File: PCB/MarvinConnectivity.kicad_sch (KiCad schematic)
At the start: 13 parts, among them J1 PROG / DBG, J10 EXP1, J11 EXP2, J2 EXPA, J3 EXPC, J4 SERVO POW 1, J5 SERVO POW 2, J6 EXPB, J7 EXPD, J8 SERVO SIG 1, J9 SERVO SIG 2

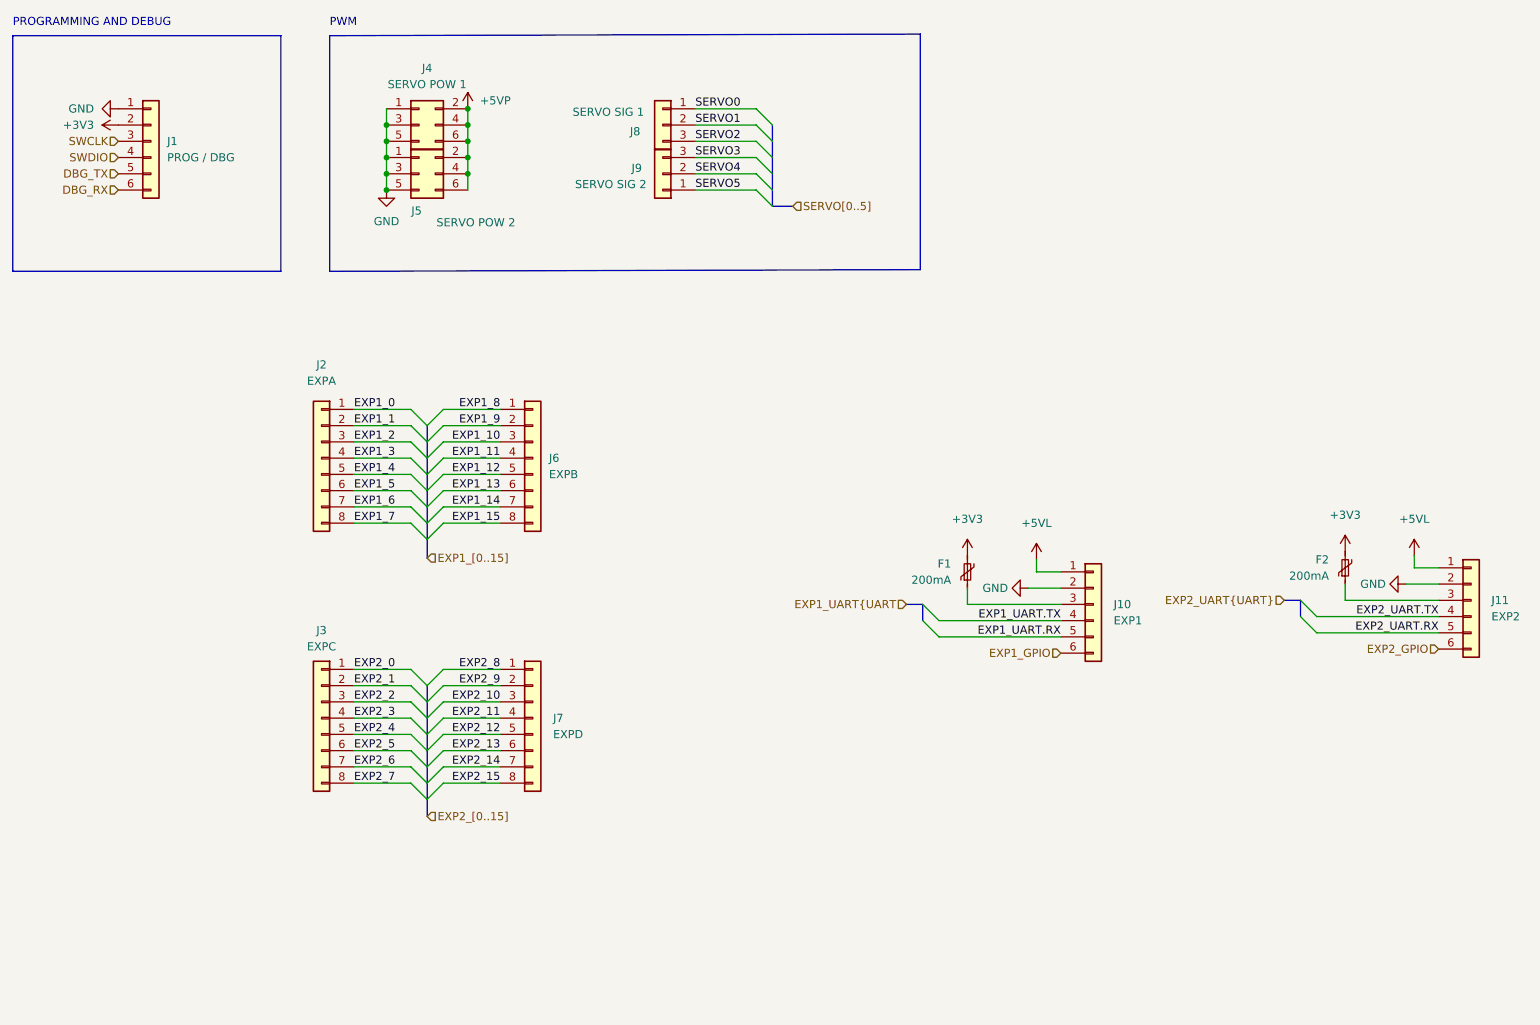
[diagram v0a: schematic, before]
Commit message: v2!
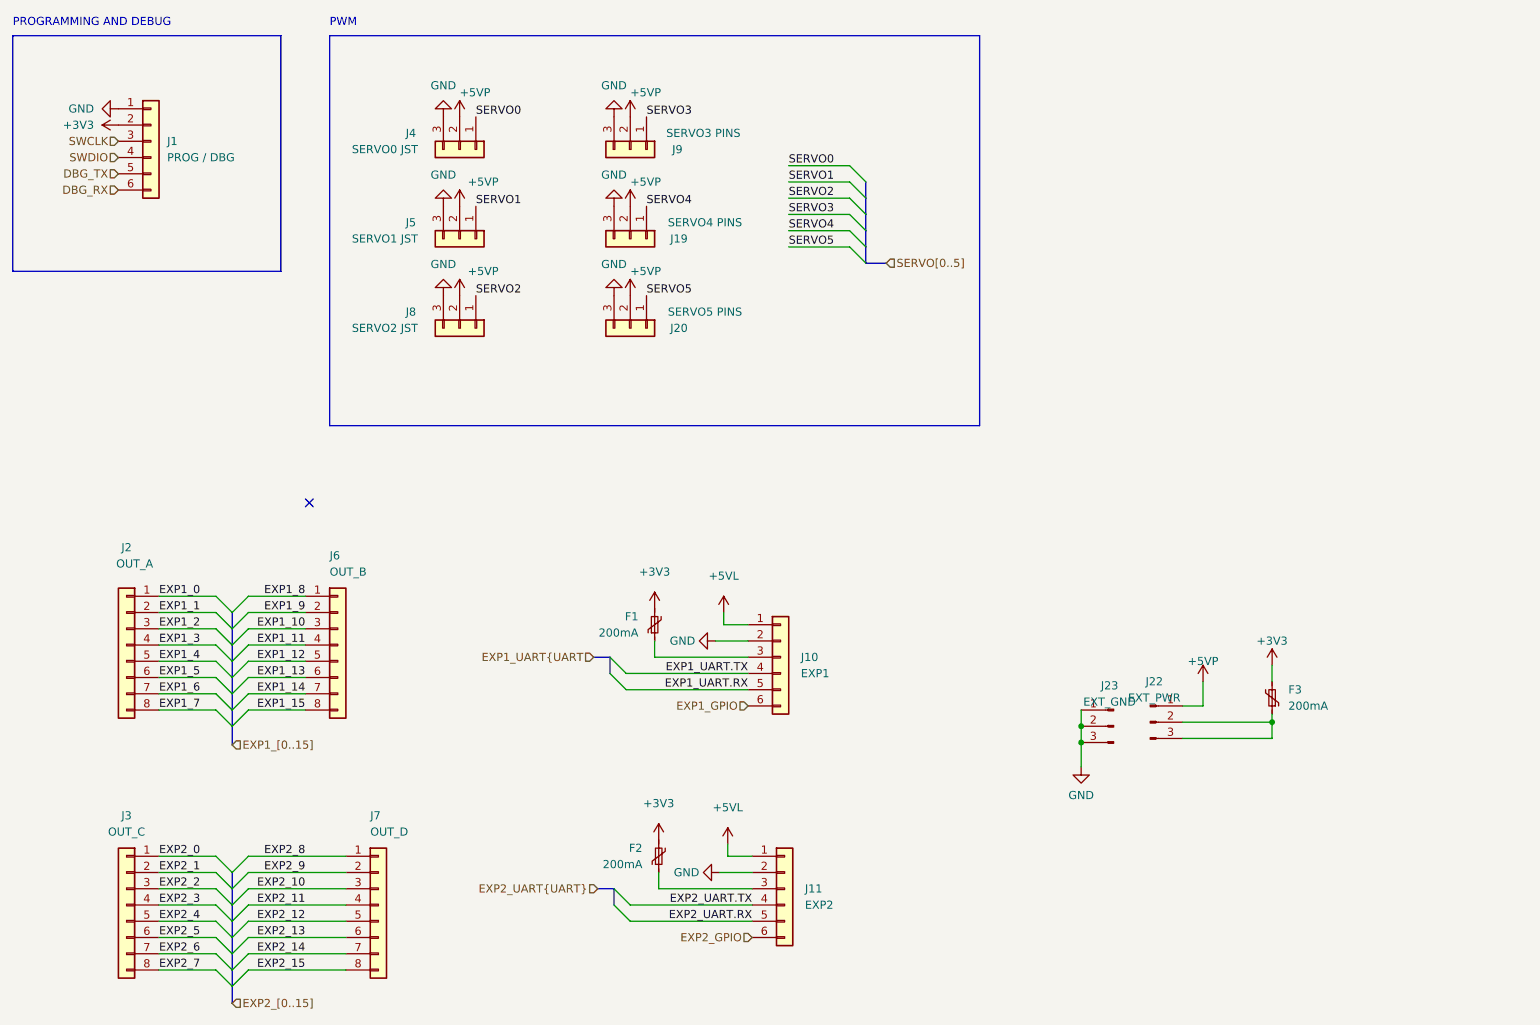
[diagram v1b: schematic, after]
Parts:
- removed J4: SERVO POW 1, Connector_PinHeader_2.54mm:PinHeader_2x03_P2.54mm_Vertical, symbol Connector_Generic:Conn_02x03_Odd_Even
- removed J5: SERVO POW 2, Connector_PinHeader_2.54mm:PinHeader_2x03_P2.54mm_Vertical, symbol Connector_Generic:Conn_02x03_Odd_Even
- added F3: 200mA, Fuse:Fuse_0603_1608Metric, symbol Device:Polyfuse_Small
- added J19: SERVO4 PINS, Connector_PinHeader_2.54mm:PinHeader_1x03_P2.54mm_Vertical, symbol Connector_Generic:Conn_01x03
- added J20: SERVO5 PINS, Connector_PinHeader_2.54mm:PinHeader_1x03_P2.54mm_Vertical, symbol Connector_Generic:Conn_01x03
- added J22: EXT_PWR, Connector_PinHeader_2.54mm:PinHeader_1x03_P2.54mm_Vertical, symbol Connector:Conn_01x03_Pin
- added J23: EXT_GND, Connector_PinHeader_2.54mm:PinHeader_1x03_P2.54mm_Vertical, symbol Connector:Conn_01x03_Pin
- added J4: SERVO0 JST, Connector_JST:JST_XH_B3B-XH-A_1x03_P2.50mm_Vertical, symbol Connector_Generic:Conn_01x03
- added J5: SERVO1 JST, Connector_JST:JST_XH_B3B-XH-A_1x03_P2.50mm_Vertical, symbol Connector_Generic:Conn_01x03
- J2: value EXPA -> OUT_A
- J3: value EXPC -> OUT_C
- J6: value EXPB -> OUT_B
- J7: value EXPD -> OUT_D
- J8: value SERVO SIG 1 -> SERVO2 JST; footprint Connector_PinHeader_2.54mm:PinHeader_1x03_P2.54mm_Vertical -> Connector_JST:JST_XH_B3B-XH-A_1x03_P2.50mm_Vertical
- J9: value SERVO SIG 2 -> SERVO3 PINS
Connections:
- net +3V3: now also F3.2
- net +5VP: now also J8.2 (Pin_2), J9.2 (Pin_2), J19.2 (Pin_2), J20.2 (Pin_2), J22.1 (Pin_1), J4.2 (Pin_2), J5.2 (Pin_2)
- net GND: now also J8.3 (Pin_3), J9.3 (Pin_3), J19.3 (Pin_3), J20.3 (Pin_3), J23.1 (Pin_1), J23.2 (Pin_2), J23.3 (Pin_3), J4.3 (Pin_3), J5.3 (Pin_3)
- net SERVO0: now also J4.1 (Pin_1); no longer J8.1 (Pin_1)
- net SERVO1: now also J5.1 (Pin_1); no longer J8.2 (Pin_2)
- net SERVO2: now also J8.1 (Pin_1); no longer J8.3 (Pin_3)
- net SERVO3: now also J9.1 (Pin_1); no longer J9.3 (Pin_3)
- net SERVO4: now also J19.1 (Pin_1); no longer J9.2 (Pin_2)
- net SERVO5: now also J20.1 (Pin_1); no longer J9.1 (Pin_1)
- new net: F3.1, J22.2 (Pin_2), J22.3 (Pin_3)
- no-connect marks 0 -> 1
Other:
- moved on the sheet: F1, F2, J10, J11, J2, J3, J6, J7
